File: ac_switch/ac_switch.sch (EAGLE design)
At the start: 7 parts, among them IC1 LM358D, T1 BC337

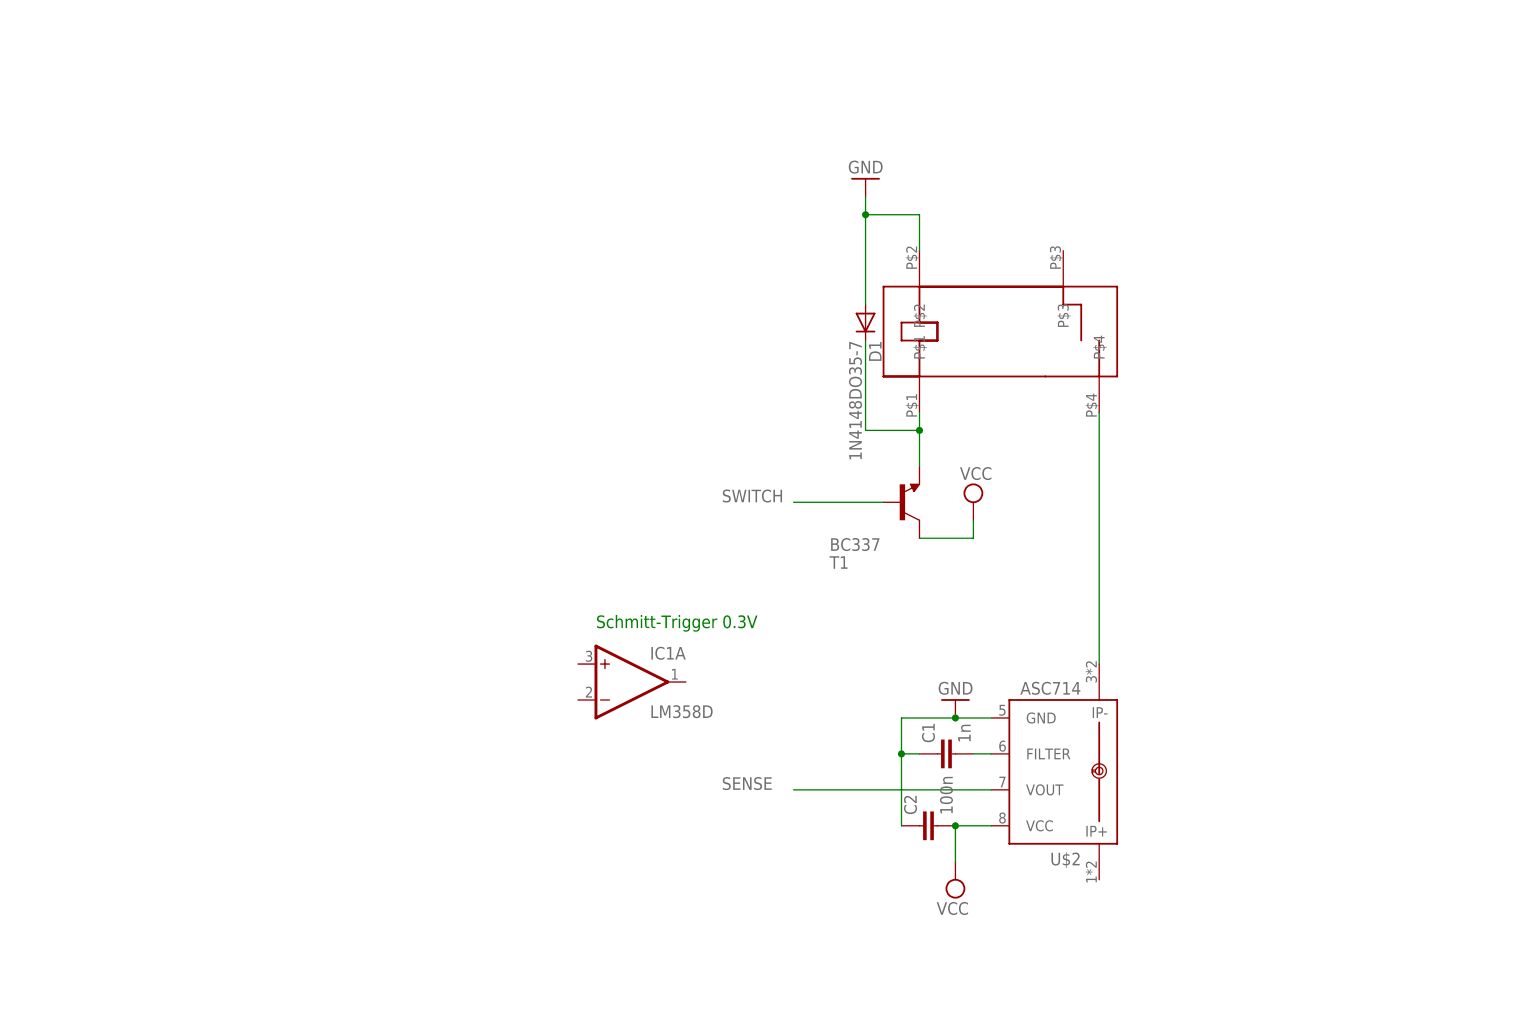
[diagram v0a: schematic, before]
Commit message: schaltung AC-Switch 98% fertig
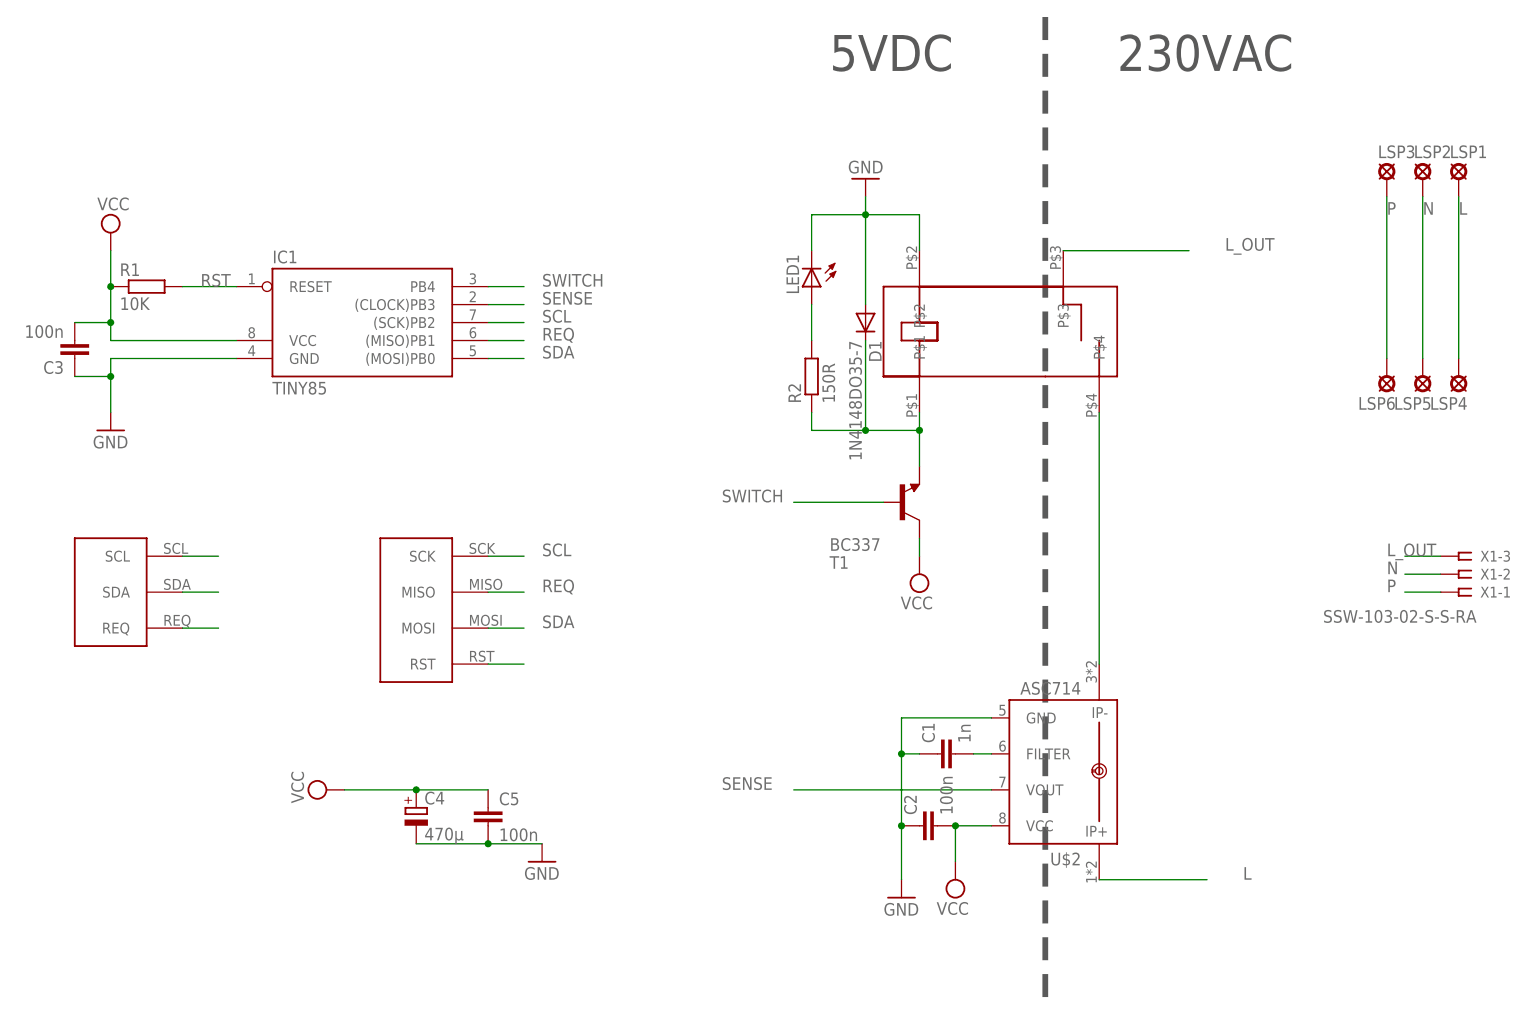
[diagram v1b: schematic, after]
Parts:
- added C3, C5: 100n, resistor:C-EU025-024X044
- added C4: 470µ, resistor:CPOL-EUE2.5-7
- added LED1: (no value), led:LED5MM
- added LSP1, LSP2, LSP3, LSP4, LSP5, LSP6: SE14, solpad:SE14
- added R1: 10K, resistor:R-EU_0207/10
- added R2: 150R, resistor:R-EU_0207/10
- added U$3: I3C_PORT, n39:I3C_PORT
- added U$4: AVR_ISP, n39:AVR_ISP
- added X1: SSW-103-02-S-S-RA, con-samtec:SSW-103-02-S-S-RA
- IC1: value LM358D -> TINY85; device linear:LM358D -> atmel:TINY22P
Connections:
- new net L: LSP1.MP, LSP4.MP, U$2.IP+
- new net L_OUT: U$1.P$3, X1-3.1
- new net N: LSP2.MP, LSP5.MP, X1-2.1
- new net N$5: LED1.A, R2.2
- new net P: LSP3.MP, LSP6.MP, X1-1.1
- new net REQ: IC1.(MISO)PB1, U$3.REQ, U$4.MISO
- new net RST: IC1.RESET, R1.2, U$4.RST
- new net SCL: IC1.(SCK)PB2, U$3.SCL, U$4.SCK
- new net SDA: IC1.(MOSI)PB0, U$3.SDA, U$4.MOSI
- net GND: now also C3.1, C4.-, C5.2, IC1.GND, LED1.C
- net N$1: now also R2.1
- net SENSE: now also IC1.(CLOCK)PB3
- net SWITCH: now also IC1.PB4
- net VCC: now also C3.2, C4.+, C5.1, IC1.VCC, R1.1
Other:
- note added: "230VAC"
- note added: "5VDC"
- note removed: "Schmitt-Trigger 0.3V"
